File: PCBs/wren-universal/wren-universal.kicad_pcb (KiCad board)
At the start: 2 copper layers, 227.7 x 112.8 mm, 120 parts, among them J1 TRRS_Jack, SW0 Reset, U1 Elite-C, U2 EGG PRO MICRO

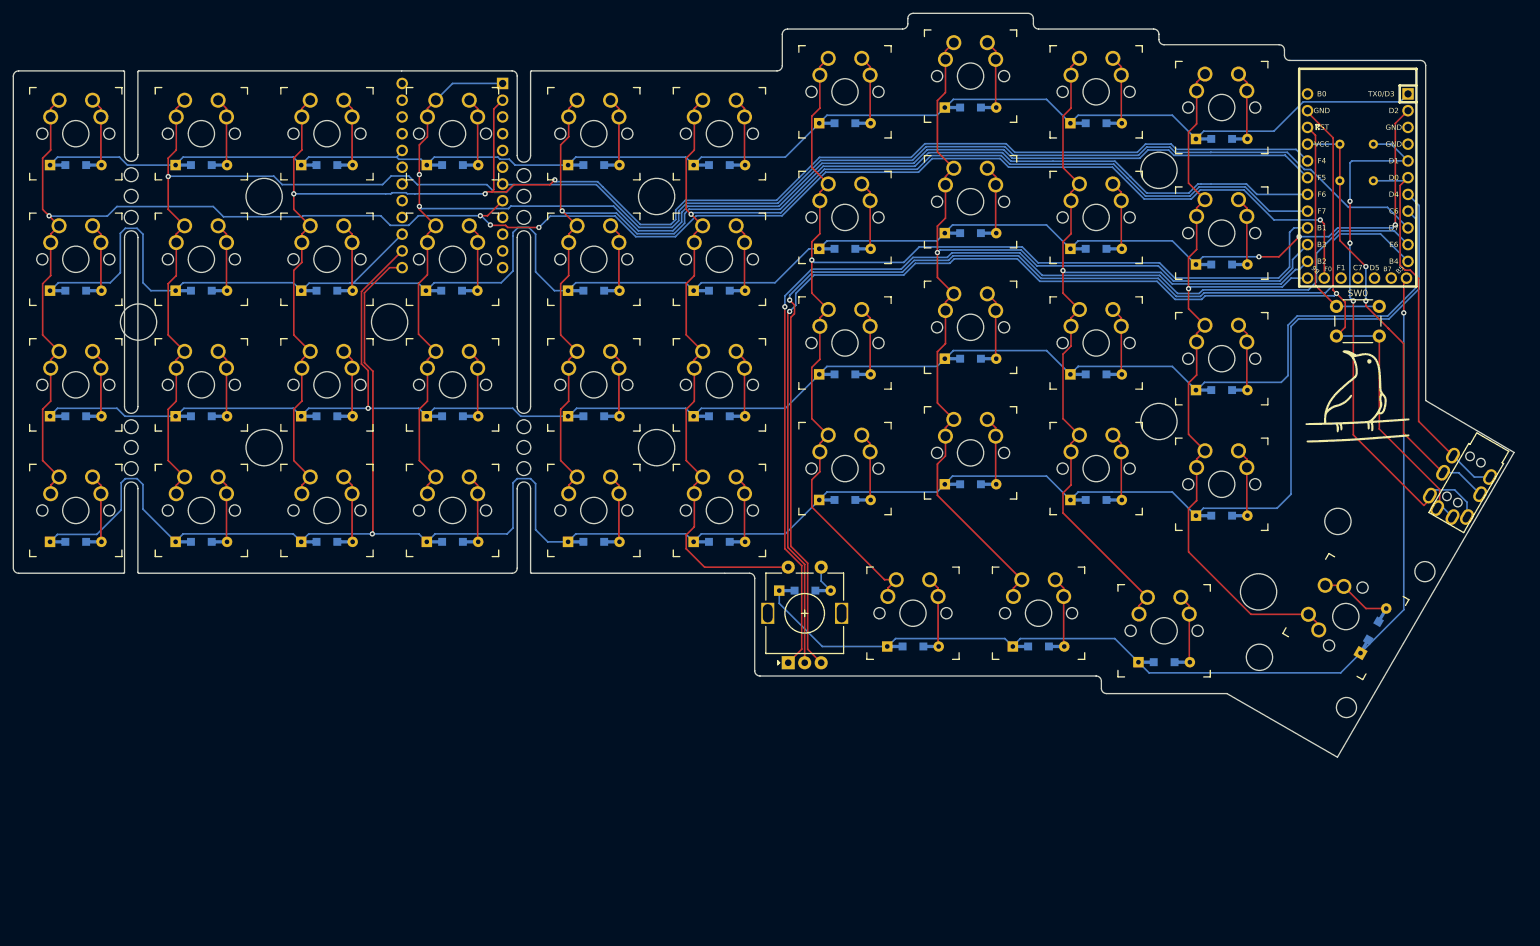
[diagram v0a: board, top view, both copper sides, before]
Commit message: Minor Changes
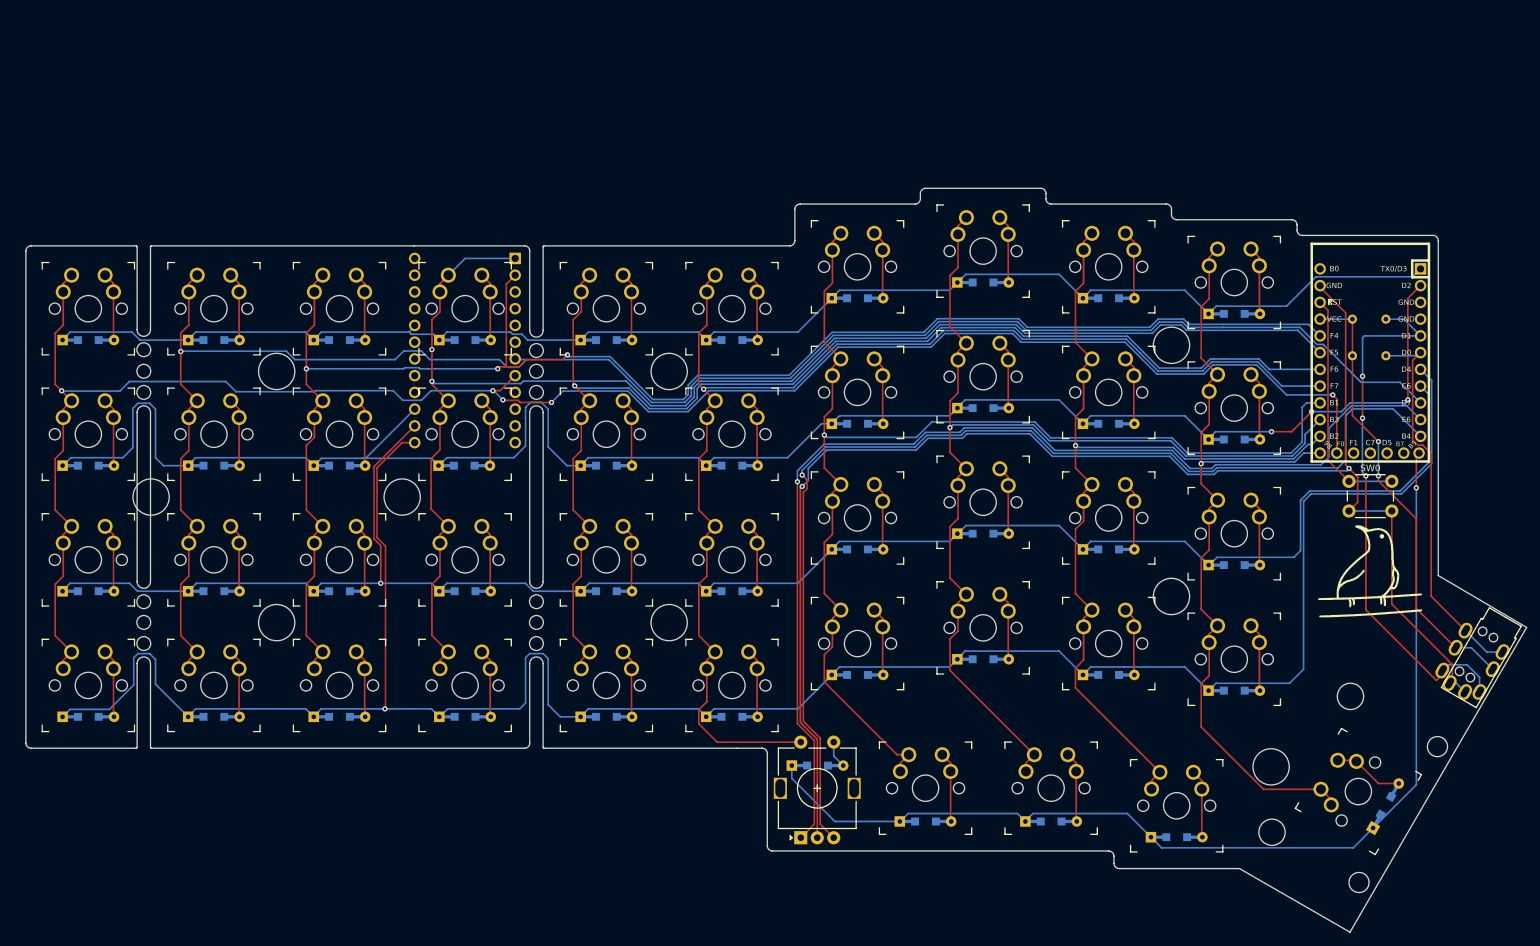
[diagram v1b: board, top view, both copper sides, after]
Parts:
- moved D13 26.6 mm to (184.5, 78.1)
- moved D2 26.6 mm to (203.5, 61.5)
- moved D21 26.6 mm to (222.6, 101.9)
- moved D23 26.6 mm to (184.5, 97.2)
- moved D25 26.6 mm to (146.4, 105.9)
- moved D26 26.6 mm to (127.3, 105.9)
- moved D27 26.6 mm to (105.9, 105.9)
- moved D28 26.6 mm to (86.8, 105.9)
- moved D29 26.6 mm to (67.8, 105.9)
- moved D30 26.6 mm to (48.7, 105.9)
- moved D31 26.6 mm to (222.6, 121.0)
- moved D33 26.6 mm to (184.5, 116.2)
- moved D35 26.6 mm to (146.4, 125.0)
- moved D36 26.6 mm to (127.3, 125.0)
- moved D37 26.6 mm to (105.9, 125.0)
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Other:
- outline, holes or cut-outs redrawn
